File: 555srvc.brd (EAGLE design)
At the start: 19.6 x 6.9 mm, 10 parts, among them IC1 555

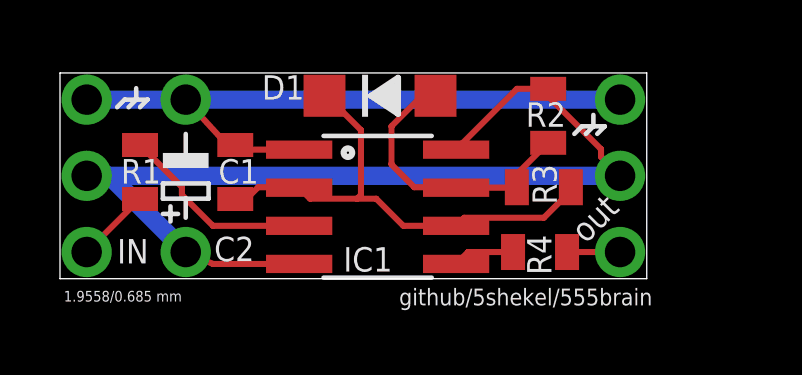
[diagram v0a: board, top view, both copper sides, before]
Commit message: update pic, and sorted silkscreen
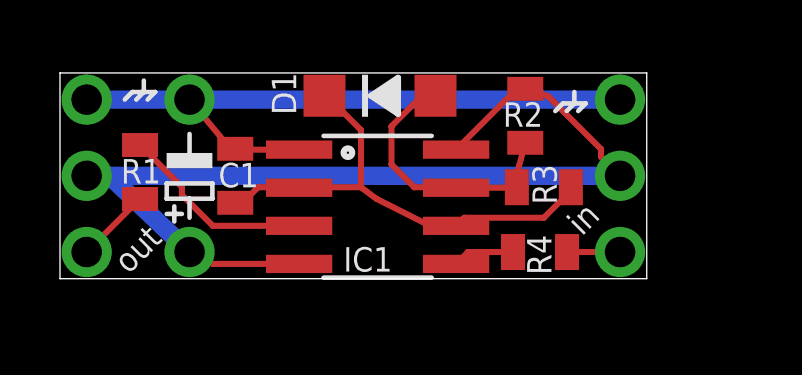
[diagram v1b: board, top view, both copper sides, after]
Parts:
- JP2: value SERVO_OUT -> servo_out
- moved R2 0.76 mm to (15.5, 5.43)
- moved C1 0.13 mm to (5.84, 3.43)
- moved C2 0.13 mm to (4.32, 3.43)
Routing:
- net N$1: track 16.5 -> 15.9 mm
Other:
- board text added: "in"
- board text removed: "IN"
